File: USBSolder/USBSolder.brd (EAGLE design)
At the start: 156.2 x 102.9 mm, 13 parts

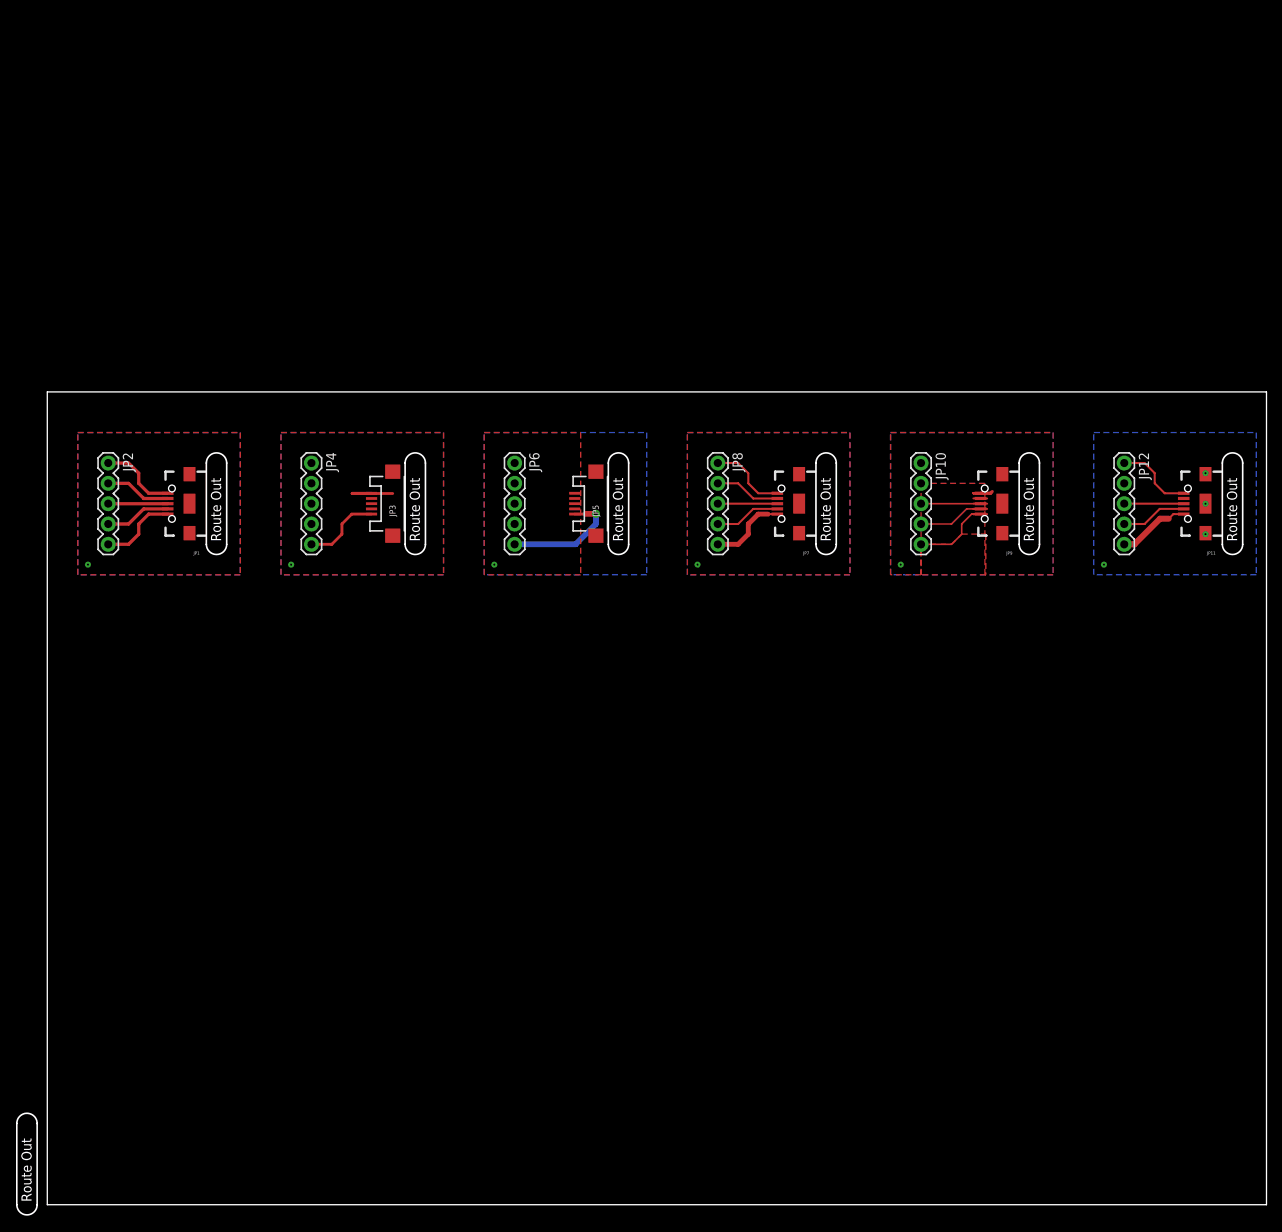
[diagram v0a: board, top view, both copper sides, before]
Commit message: done with usb test
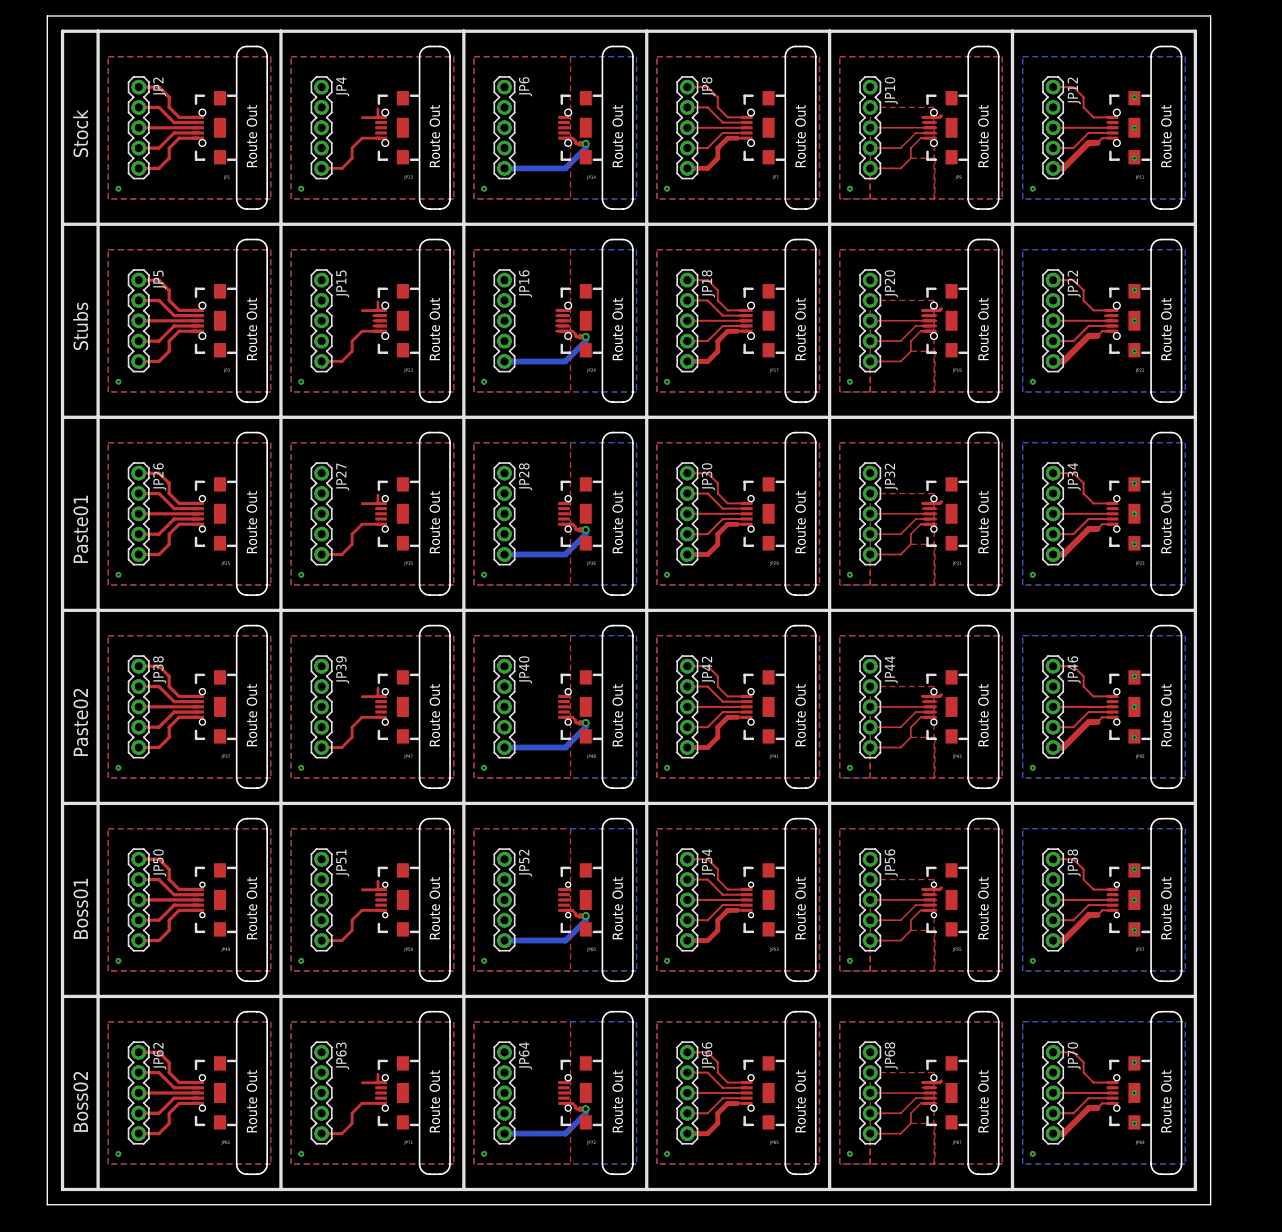
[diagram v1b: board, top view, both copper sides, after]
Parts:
- added JP13, JP14: (no value), TestUSBs:USB-B-MICRO-SMD_V03
- added JP15, JP16, JP18, JP20, JP22, JP26, JP27, JP28, JP30, JP32, JP34, JP38, JP39, JP40, JP42, JP44, JP46, JP50, JP51, JP52, JP54, JP56, JP58, JP62, JP63, JP64, JP66, JP68, JP70: (no value), SparkFun-Connectors:1X05
- added JP17, JP19, JP21, JP23, JP24: (no value), TestUSBs:USB-MICRO-STUBS-01
- added JP25, JP29, JP31, JP33, JP35, JP36: (no value), TestUSBs:USB-MICRO-PASTE-01
- added JP37, JP41, JP43, JP45, JP47, JP48: (no value), TestUSBs:USB-MICRO-PASTE-02
- added JP49, JP53, JP55, JP57, JP59, JP60: (no value), TestUSBs:USB-MICRO-BOSS-01
- added JP61, JP65, JP67, JP69, JP71, JP72: (no value), TestUSBs:USB-MICRO-BOSS-02
- JP1, JP11, JP7, JP9: device SparkFun-Connectors:USB-B-MICRO-SMD_V03 -> TestUSBs:USB-B-MICRO-SMD_V03
- JP3: device TestUSBs:CHARGERS -> TestUSBs:USB-MICRO-STUBS-01
- JP5: device TestUSBs:CHARGERS -> SparkFun-Connectors:1X05
- moved JP5 63.6 mm to (11.4, 115.6), turned to 270 degrees
- moved JP11 47.8 mm to (135.9, 134.6)
- moved JP12 47.8 mm to (125.7, 139.7)
- moved JP9 47.4 mm to (113.0, 134.6)
- moved JP10 47.4 mm to (102.9, 139.7)
- moved JP1 47.1 mm to (21.6, 134.6)
- moved JP7 47.1 mm to (90.2, 134.6)
- moved JP2 47.1 mm to (11.4, 139.7)
- moved JP8 47.1 mm to (80.0, 139.7)
- moved JP4 47.0 mm to (34.3, 139.7)
- moved JP6 47.0 mm to (57.1, 139.7)
- moved JP3 31.4 mm to (21.6, 110.5), turned to 180 degrees
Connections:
- new net 5V2: JP16.5, JP24.VBUS1
- new net 5V3: JP28.5, JP36.VBUS1
- new net 5V4: JP40.5, JP48.VBUS1
- new net 5V5: JP52.5, JP60.VBUS1
- new net 5V6: JP64.5, JP72.VBUS1
- new net GND1: JP15.1, JP16.1, JP17.GND1, JP18.1, JP19.GND1, JP20.1, JP21.GND1, JP21.SHIELD1, JP21.SHIELD2, JP21.SHIELD3, JP22.1, JP23.GND1, JP24.GND1, JP3.SHIELD1, JP3.SHIELD2, JP3.SHIELD3
- new net GND2: JP25.SHIELD1, JP25.SHIELD2, JP25.SHIELD3, JP27.1, JP28.1, JP29.GND1, JP30.1, JP31.GND1, JP32.1, JP33.GND1, JP33.SHIELD1, JP33.SHIELD2, JP33.SHIELD3, JP34.1, JP35.GND1, JP36.GND1
- new net GND3: JP37.SHIELD1, JP37.SHIELD2, JP37.SHIELD3, JP39.1, JP40.1, JP41.GND1, JP42.1, JP43.GND1, JP44.1, JP45.GND1, JP45.SHIELD1, JP45.SHIELD2, JP45.SHIELD3, JP46.1, JP47.GND1, JP48.GND1
- new net GND4: JP49.SHIELD1, JP49.SHIELD2, JP49.SHIELD3, JP51.1, JP52.1, JP53.GND1, JP54.1, JP55.GND1, JP56.1, JP57.GND1, JP57.SHIELD1, JP57.SHIELD2, JP57.SHIELD3, JP58.1, JP59.GND1, JP60.GND1
- new net GND5: JP61.SHIELD1, JP61.SHIELD2, JP61.SHIELD3, JP63.1, JP64.1, JP65.GND1, JP66.1, JP67.GND1, JP68.1, JP69.GND1, JP69.SHIELD1, JP69.SHIELD2, JP69.SHIELD3, JP70.1, JP71.GND1, JP72.GND1
- new net N$100: JP69.D-1, JP70.4
- new net N$101: JP69.VBUS1, JP70.5
- new net N$14: JP3.D+1, JP5.3
- new net N$15: JP3.D-1, JP5.4
- new net N$19: JP3.VBUS1, JP5.5
- new net N$20: JP15.5, JP23.VBUS1
- new net N$24: JP17.ID1, JP18.2
- new net N$25: JP17.D+1, JP18.3
- new net N$26: JP17.D-1, JP18.4
- new net N$27: JP17.VBUS1, JP18.5
- new net N$28: JP19.D+1, JP20.3
- new net N$29: JP19.D-1, JP20.4
- new net N$30: JP19.VBUS1, JP20.5
- new net N$31: JP21.D+1, JP22.3
- new net N$32: JP21.D-1, JP22.4
- new net N$33: JP21.VBUS1, JP22.5
- new net N$35: JP25.GND1, JP26.1
- new net N$36: JP25.ID1, JP26.2
- new net N$37: JP25.D+1, JP26.3
- new net N$38: JP25.D-1, JP26.4
- new net N$39: JP25.VBUS1, JP26.5
- new net N$40: JP27.5, JP35.VBUS1
- new net N$41: JP29.ID1, JP30.2
- new net N$42: JP29.D+1, JP30.3
- new net N$43: JP29.D-1, JP30.4
- new net N$44: JP29.VBUS1, JP30.5
- new net N$45: JP31.D+1, JP32.3
- new net N$46: JP31.D-1, JP32.4
- new net N$47: JP31.VBUS1, JP32.5
- new net N$48: JP33.D+1, JP34.3
- new net N$49: JP33.D-1, JP34.4
- new net N$50: JP33.VBUS1, JP34.5
- new net N$52: JP37.GND1, JP38.1
- new net N$53: JP37.ID1, JP38.2
- new net N$54: JP37.D+1, JP38.3
- new net N$55: JP37.D-1, JP38.4
- new net N$56: JP37.VBUS1, JP38.5
- new net N$57: JP39.5, JP47.VBUS1
- new net N$58: JP41.ID1, JP42.2
- new net N$59: JP41.D+1, JP42.3
- new net N$60: JP41.D-1, JP42.4
- new net N$61: JP41.VBUS1, JP42.5
- new net N$62: JP43.D+1, JP44.3
- new net N$63: JP43.D-1, JP44.4
- new net N$64: JP43.VBUS1, JP44.5
- new net N$65: JP45.D+1, JP46.3
- new net N$66: JP45.D-1, JP46.4
- new net N$67: JP45.VBUS1, JP46.5
- new net N$69: JP49.GND1, JP50.1
- new net N$7: JP3.GND1, JP5.1
- new net N$70: JP49.ID1, JP50.2
- new net N$71: JP49.D+1, JP50.3
- new net N$72: JP49.D-1, JP50.4
- new net N$73: JP49.VBUS1, JP50.5
- new net N$74: JP51.5, JP59.VBUS1
- new net N$75: JP53.ID1, JP54.2
- new net N$76: JP53.D+1, JP54.3
- new net N$77: JP53.D-1, JP54.4
- new net N$78: JP53.VBUS1, JP54.5
- new net N$79: JP55.D+1, JP56.3
- new net N$8: JP3.ID1, JP5.2
- new net N$80: JP55.D-1, JP56.4
- new net N$81: JP55.VBUS1, JP56.5
- new net N$82: JP57.D+1, JP58.3
- new net N$83: JP57.D-1, JP58.4
- new net N$84: JP57.VBUS1, JP58.5
- new net N$86: JP61.GND1, JP62.1
- new net N$87: JP61.ID1, JP62.2
- new net N$88: JP61.D+1, JP62.3
- new net N$89: JP61.D-1, JP62.4
- new net N$90: JP61.VBUS1, JP62.5
- new net N$91: JP63.5, JP71.VBUS1
- new net N$92: JP65.ID1, JP66.2
- new net N$93: JP65.D+1, JP66.3
- new net N$94: JP65.D-1, JP66.4
- new net N$95: JP65.VBUS1, JP66.5
- new net N$96: JP67.D+1, JP68.3
- new net N$97: JP67.D-1, JP68.4
- new net N$98: JP67.VBUS1, JP68.5
- new net N$99: JP69.D+1, JP70.3
- net 5V1: now also JP14.VBUS1; no longer JP5.VBUS
- net GND: now also JP13.GND1, JP14.GND1; no longer JP3.GND, JP5.GND
- net N$10: now also JP13.VBUS1; no longer JP3.VBUS
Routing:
- net GND4: track 0.00 -> 28.1 mm, vias 0 -> 9
- net GND3: track 0.00 -> 28.1 mm, vias 0 -> 9
- net GND2: track 0.00 -> 28.1 mm, vias 0 -> 9
- net GND5: track 0.00 -> 28.1 mm, vias 0 -> 9
- net GND1: track 0.00 -> 28.1 mm, vias 0 -> 9
- net 5V3: track 0.00 -> 14.9 mm, vias 0 -> 1
- net 5V6: track 0.00 -> 14.9 mm, vias 0 -> 1
- net 5V2: track 0.00 -> 14.9 mm, vias 0 -> 1
- net 5V4: track 0.00 -> 14.9 mm, vias 0 -> 1
- net 5V5: track 0.00 -> 14.9 mm, vias 0 -> 1
- net N$98: track 0.00 -> 12.3 mm
- net N$64: track 0.00 -> 12.3 mm
- net N$47: track 0.00 -> 12.3 mm
- net N$30: track 0.00 -> 12.3 mm
- net N$81: track 0.00 -> 12.3 mm
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- added copper zone on layer 1, net GND1
- added copper zone on layer 16, net GND1
- added copper zone on layer 1, net GND2
- added copper zone on layer 16, net GND2
- added copper zone on layer 1, net GND3
- added copper zone on layer 16, net GND3
- added copper zone on layer 1, net GND4
- added copper zone on layer 16, net GND4
- added copper zone on layer 1, net GND5
- added copper zone on layer 16, net GND5
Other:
- board size 156.2 x 102.9 mm -> 145.4 x 148.6 mm
- board text added: "Boss01"
- board text added: "Boss02"
- board text added: "Paste01"
- board text added: "Paste02"
- board text added: "Stock"
- board text added: "Stubs"
